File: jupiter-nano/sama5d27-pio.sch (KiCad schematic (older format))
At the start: 1 part, among them U1 ATSAMA5D27C-LD1G-CU

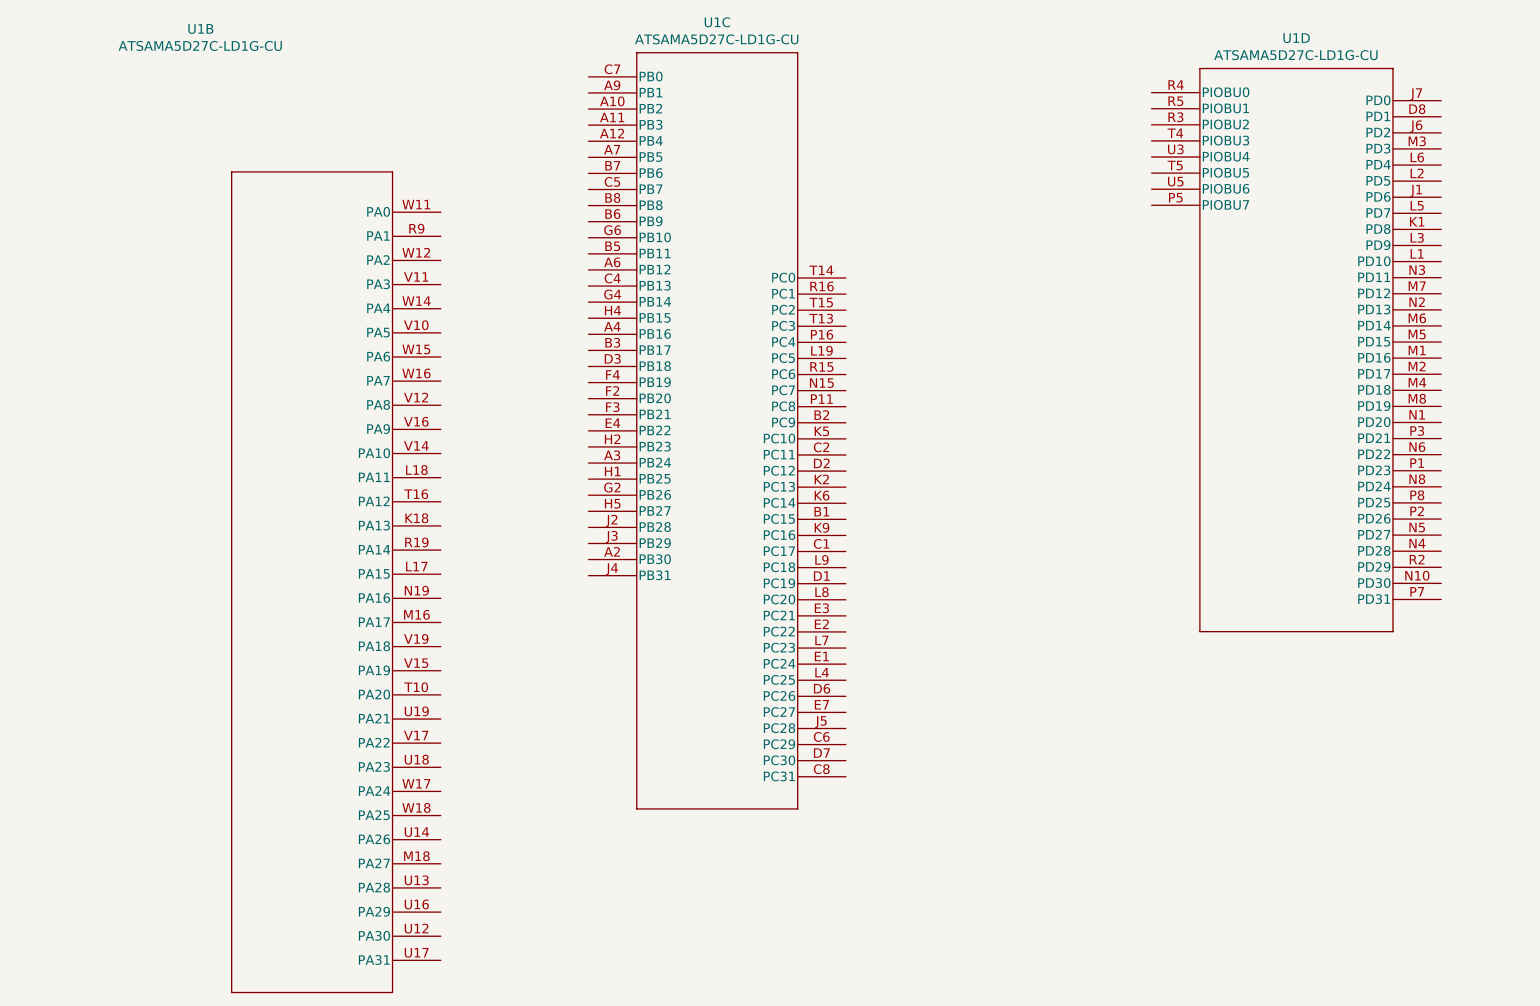
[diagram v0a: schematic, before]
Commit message: WIP, PIO done
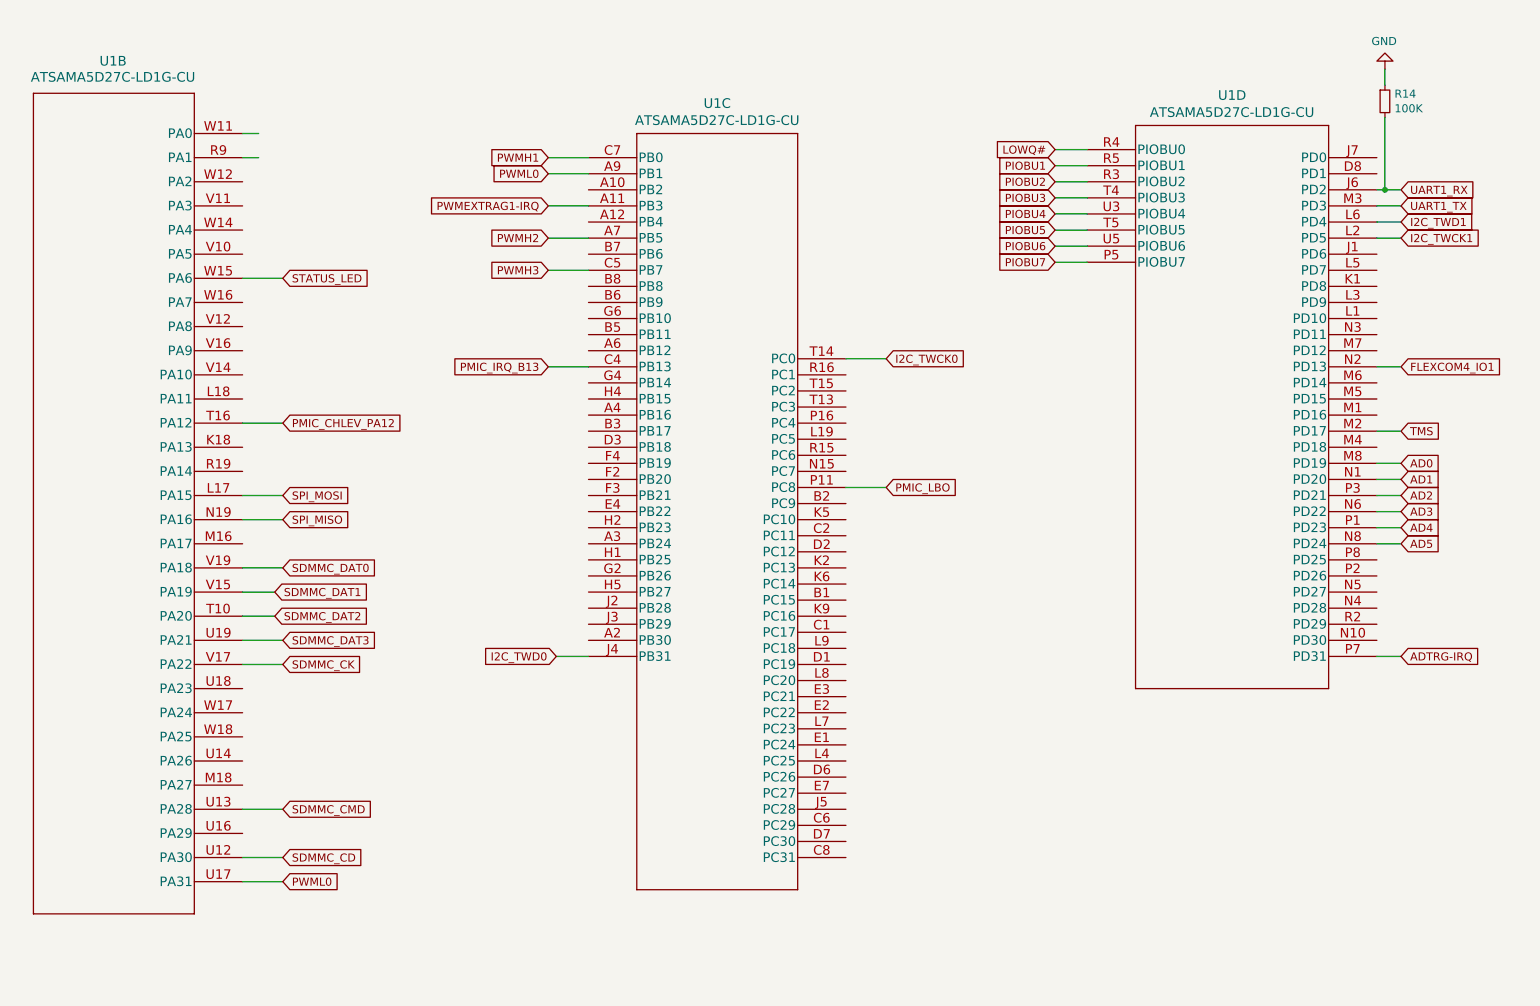
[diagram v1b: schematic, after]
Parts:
- added R14: 100K, symbol Device:R_Small
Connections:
- net labels added: AD0, AD1, AD2, AD3, AD4, AD5, ADTRG-IRQ, FLEXCOM4_IO1, GND, I2C_TWCK0, I2C_TWCK1, I2C_TWD0, I2C_TWD1, LOWQ#, PIOBU1, PIOBU2, PIOBU3, PIOBU4, PIOBU5, PIOBU6, PIOBU7, PMIC_CHLEV_PA12, PMIC_IRQ_B13, PMIC_LBO, PWMEXTRAG1-IRQ, PWMH1, PWMH2, PWMH3, PWML0, SDMMC_CD, SDMMC_CK, SDMMC_CMD, SDMMC_DAT0, SDMMC_DAT1, SDMMC_DAT2, SDMMC_DAT3, SPI_MISO, SPI_MOSI, STATUS_LED, TMS, UART1_RX, UART1_TX
- wire segments 0 -> 47
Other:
- moved on the sheet: U1B, U1C, U1D
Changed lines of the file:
@@
 L ATSAMA5D27C-LD1G:ATSAMA5D27C-LD1G-CU U1
 U 2 1 5F5990A8
-P 2382 1089
-F 0 "U1" H 1740 1576 60  0000 C CNN
-F 1 "ATSAMA5D27C-LD1G-CU" H 1740 1470 60  0000 C CNN
-F 2 "TFBGA361_16X16_MCH" H 3582 1429 60  0001 C CNN
-F 3 "" H 2382 1089 60  0000 C CNN
-	2    2382 1089
-	1    0    0    -1
-$EndComp
+P 1150 600
+F 0 "U1" H 1195 400 60  0000 C CNN
+F 1 "ATSAMA5D27C-LD1G-CU" H 1195 300 60  0000 C CNN
+F 2 "TFBGA361_16X16_MCH" H 2350 940 60  0001 C CNN
+F 3 "" H 1150 600 60  0000 C CNN
+	2    1150 600
+	1    0    0    -1
+$EndComp
+$Comp
+L ATSAMA5D27C-LD1G:ATSAMA5D27C-LD1G-CU U1
+U 4 1 5F5C0676
+P 7250 1400
+F 0 "U1" H 8150 1787 60  0000 C CNN
+F 1 "ATSAMA5D27C-LD1G-CU" H 8150 1681 60  0000 C CNN
+F 2 "TFBGA361_16X16_MCH" H 8450 1740 60  0001 C CNN
+F 3 "" H 7250 1400 60  0000 C CNN
+	4    7250 1400
+	1    0    0    -1
+$EndComp
+Wire Wire Line
+	2000 2150 2250 2150
+Text GLabel 2250 2150 2    50   Input ~ 0
+STATUS_LED
+Text GLabel 2250 3050 2    50   Input ~ 0
+PMIC_CHLEV_PA12
+Text GLabel 2250 3500 2    50   Input ~ 0
+SPI_MOSI
+Text GLabel 2250 3650 2    50   Input ~ 0
+SPI_MISO
+Text GLabel 2250 3950 2    50   Input ~ 0
+SDMMC_DAT0
+Text GLabel 2200 4100 2    50   Input ~ 0
+SDMMC_DAT1
+Text GLabel 2200 4250 2    50   Input ~ 0
+SDMMC_DAT2
+Text GLabel 2250 4400 2    50   Input ~ 0
+SDMMC_DAT3
+Text GLabel 2250 4550 2    50   Input ~ 0
+SDMMC_CK
+Text GLabel 2250 5450 2    50   Input ~ 0
+SDMMC_CMD
+Text GLabel 2250 5750 2    50   Input ~ 0
+SDMMC_CD
+Text GLabel 2250 5900 2    50   Input ~ 0
+PWML0
+Text GLabel 3900 1500 0    50   Input ~ 0
+PWML0
+Wire Wire Line
+	2000 3050 2250 3050
+Wire Wire Line
+	2000 3500 2250 3500
+Wire Wire Line
+	2000 3650 2250 3650
 $Comp
 L ATSAMA5D27C-LD1G:ATSAMA5D27C-LD1G-CU U1
 U 3 1 5F5A7AFC
-P 4150 948
-F 0 "U1" H 4950 1335 60  0000 C CNN
-F 1 "ATSAMA5D27C-LD1G-CU" H 4950 1229 60  0000 C CNN
-F 2 "TFBGA361_16X16_MCH" H 5350 1288 60  0001 C CNN
-F 3 "" H 4150 948 60  0000 C CNN
-	3    4150 948
-	1    0    0    -1
-$EndComp
-$Comp
-L ATSAMA5D27C-LD1G:ATSAMA5D27C-LD1G-CU U1
-U 4 1 5F5C0676
-P 7650 1046
-F 0 "U1" H 8550 1433 60  0000 C CNN
-F 1 "ATSAMA5D27C-LD1G-CU" H 8550 1327 60  0000 C CNN
-F 2 "TFBGA361_16X16_MCH" H 8850 1386 60  0001 C CNN
-F 3 "" H 7650 1046 60  0000 C CNN
-	4    7650 1046
-	1    0    0    -1
+P 4150 1450
+F 0 "U1" H 4950 1837 60  0000 C CNN
+F 1 "ATSAMA5D27C-LD1G-CU" H 4950 1731 60  0000 C CNN
+F 2 "TFBGA361_16X16_MCH" H 5350 1790 60  0001 C CNN
+F 3 "" H 4150 1450 60  0000 C CNN
+	3    4150 1450
+	1    0    0    -1
+$EndComp
+Wire Wire Line
+	2000 1250 2100 1250
+Wire Wire Line
+	2000 1400 2100 1400
+Wire Wire Line
+	4150 1400 3900 1400
+Wire Wire Line
+	3900 1500 4150 1500
+Wire Wire Line
+	2000 3950 2250 3950
+Wire Wire Line
+	2000 4100 2200 4100
+Wire Wire Line
+	2000 4250 2200 4250
+Wire Wire Line
+	2000 4400 2250 4400
+Wire Wire Line
+	2000 4550 2250 4550
+Wire Wire Line
+	2000 5450 2250 5450
+Wire Wire Line
+	2000 5750 2250 5750
+Wire Wire Line
+	2000 5900 2250 5900
+Text GLabel 3900 1400 0    50   Input ~ 0
+PWMH1
+Text GLabel 3900 1700 0    50   Input ~ 0
+PWMEXTRAG1-IRQ
+Text GLabel 3900 1900 0    50   Input ~ 0
+PWMH2
+Text GLabel 3900 2100 0    50   Input ~ 0
+PWMH3
+Wire Wire Line
+	3900 1700 4150 1700
+Wire Wire Line
+	3900 1900 4150 1900
+Wire Wire Line
+	3900 2100 4150 2100
+Text GLabel 3900 2700 0    50   Input ~ 0
+PMIC_IRQ_B13
+Text GLabel 3950 4500 0    50   Input ~ 0
+I2C_TWD0
+Wire Wire Line
+	3950 4500 4150 4500
+Wire Wire Line
+	3900 2700 4150 2700
+Wire Wire Line
+	5750 2650 6000 2650
+Text GLabel 6000 2650 2    50   Input ~ 0
+I2C_TWCK0
+Wire Wire Line
+	5750 3450 6000 3450
+Text GLabel 6000 3450 2    50   Input ~ 0
+PMIC_LBO
+Wire Wire Line
+	7250 1350 7050 1350
+Wire Wire Line
+	7250 1450 7050 1450
+Wire Wire Line
+	7250 1550 7050 1550
+Wire Wire Line
+	7250 1650 7050 1650
+Wire Wire Line
+	7250 1750 7050 1750
+Wire Wire Line
+	7250 1850 7050 1850
+Wire Wire Line
+	7250 1950 7050 1950
+Wire Wire Line
+	7250 2050 7050 2050
+Text GLabel 7050 1350 0    50   Input ~ 0
+LOWQ#
+Text GLabel 7050 1450 0    50   Input ~ 0
+PIOBU1
+Text GLabel 7050 1550 0    50   Input ~ 0
+PIOBU2
+Text GLabel 7050 1650 0    50   Input ~ 0
+PIOBU3
+Text GLabel 7050 1750 0    50   Input ~ 0
+PIOBU4
+Text GLabel 7050 1850 0    50   Input ~ 0
+PIOBU5
+Text GLabel 7050 1950 0    50   Input ~ 0
+PIOBU6
+Text GLabel 7050 2050 0    50   Input ~ 0
+PIOBU7
+Wire Wire Line
+	9050 1600 9100 1600
+Text GLabel 9200 1600 2    50   Input ~ 0
+UART1_RX
+Wire Wire Line
+	9050 1700 9200 1700
+Text GLabel 9200 1700 2    50   Input ~ 0
+UART1_TX
+Wire Wire Line
+	9050 1800 9200 1800
+Wire Wire Line
+	9050 1900 9200 1900
+Text GLabel 9200 1800 2    50   Input ~ 0
+I2C_TWD1
+Text GLabel 9200 1900 2    50   Input ~ 0
+I2C_TWCK1
+Wire Wire Line
+	9050 2700 9200 2700
+Wire Wire Line
+	9050 3100 9200 3100
+Wire Wire Line
+	9050 3300 9200 3300
+Wire Wire Line
+	9050 3400 9200 3400
+Wire Wire Line
+	9050 3500 9200 3500
+Wire Wire Line
+	9050 3600 9200 3600
+Wire Wire Line
+	9050 3700 9200 3700
+Wire Wire Line
+	9050 3800 9200 3800
+Text GLabel 9200 2700 2    50   Input ~ 0
+FLEXCOM4_IO1
+Text GLabel 9200 3100 2    50   Input ~ 0
+TMS
+Text GLabel 9200 3300 2    50   Input ~ 0
+AD0
+Text GLabel 9200 3400 2    50   Input ~ 0
+AD1
+Text GLabel 9200 3500 2    50   Input ~ 0
+AD2
+Text GLabel 9200 3600 2    50   Input ~ 0
+AD3
+Text GLabel 9200 3700 2    50   Input ~ 0
+AD4
+Text GLabel 9200 3800 2    50   Input ~ 0
+AD5
+Wire Wire Line
+	9050 4500 9200 4500
+Text GLabel 9200 4500 2    50   Input ~ 0
+ADTRG-IRQ
+$Comp
+L Device:R_Small R14
+U 1 1 600D6DFE
+P 9100 1050
+F 0 "R14" H 9159 1096 50  0000 L CNN
+F 1 "100K" H 9159 1005 50  0000 L CNN
+F 2 "" H 9100 1050 50  0001 C CNN
+F 3 "~" H 9100 1050 50  0001 C CNN
+	1    9100 1050
+	1    0    0    -1
+$EndComp
+Wire Wire Line
+	9100 1150 9100 1600
+Connection ~ 9100 1600
+Wire Wire Line
+	9100 1600 9200 1600
+Wire Wire Line
+	9100 950  9100 850
+$Comp
+L power:GND #PWR?
+U 1 1 600DB627
+P 9100 850
+F 0 "#PWR?" H 9100 600 50  0001 C CNN
+F 1 "GND" H 9105 677 50  0000 C CNN
+F 2 "" H 9100 850 50  0001 C CNN
+F 3 "" H 9100 850 50  0001 C CNN
+	1    9100 850
+	-1   0    0    1
 $EndComp
 $EndSCHEMATC

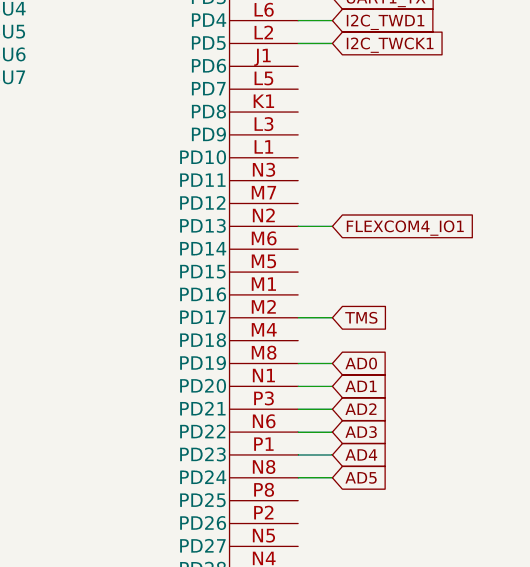
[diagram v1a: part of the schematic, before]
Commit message: WIP, USB-UART and JTAG done
- minor clean up and SD Card form factor still left
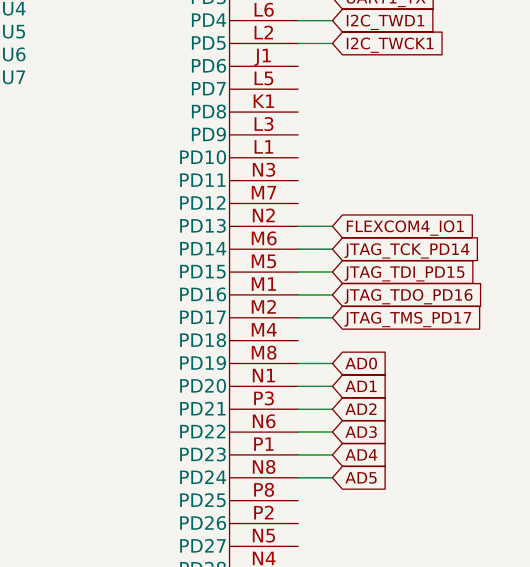
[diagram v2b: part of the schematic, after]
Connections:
- net labels added: JTAG_TCK_PD14, JTAG_TDI_PD15, JTAG_TDO_PD16, JTAG_TMS_PD17
- net labels removed: TMS
- wire segments 47 -> 50
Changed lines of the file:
@@
 FLEXCOM4_IO1
 Text GLabel 9200 3100 2    50   Input ~ 0
-TMS
+JTAG_TMS_PD17
 Text GLabel 9200 3300 2    50   Input ~ 0
 AD0
@@
 	-1   0    0    1
 $EndComp
+Wire Wire Line
+	9050 2800 9200 2800
+Wire Wire Line
+	9050 3000 9200 3000
+Wire Wire Line
+	9050 2900 9200 2900
+Text GLabel 9200 3000 2    50   Input ~ 0
+JTAG_TDO_PD16
+Text GLabel 9200 2900 2    50   Input ~ 0
+JTAG_TDI_PD15
+Text GLabel 9200 2800 2    50   Input ~ 0
+JTAG_TCK_PD14
 $EndSCHEMATC
